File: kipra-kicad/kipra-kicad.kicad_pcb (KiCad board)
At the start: 2 copper layers, 128.2 x 134.8 mm, 51 parts

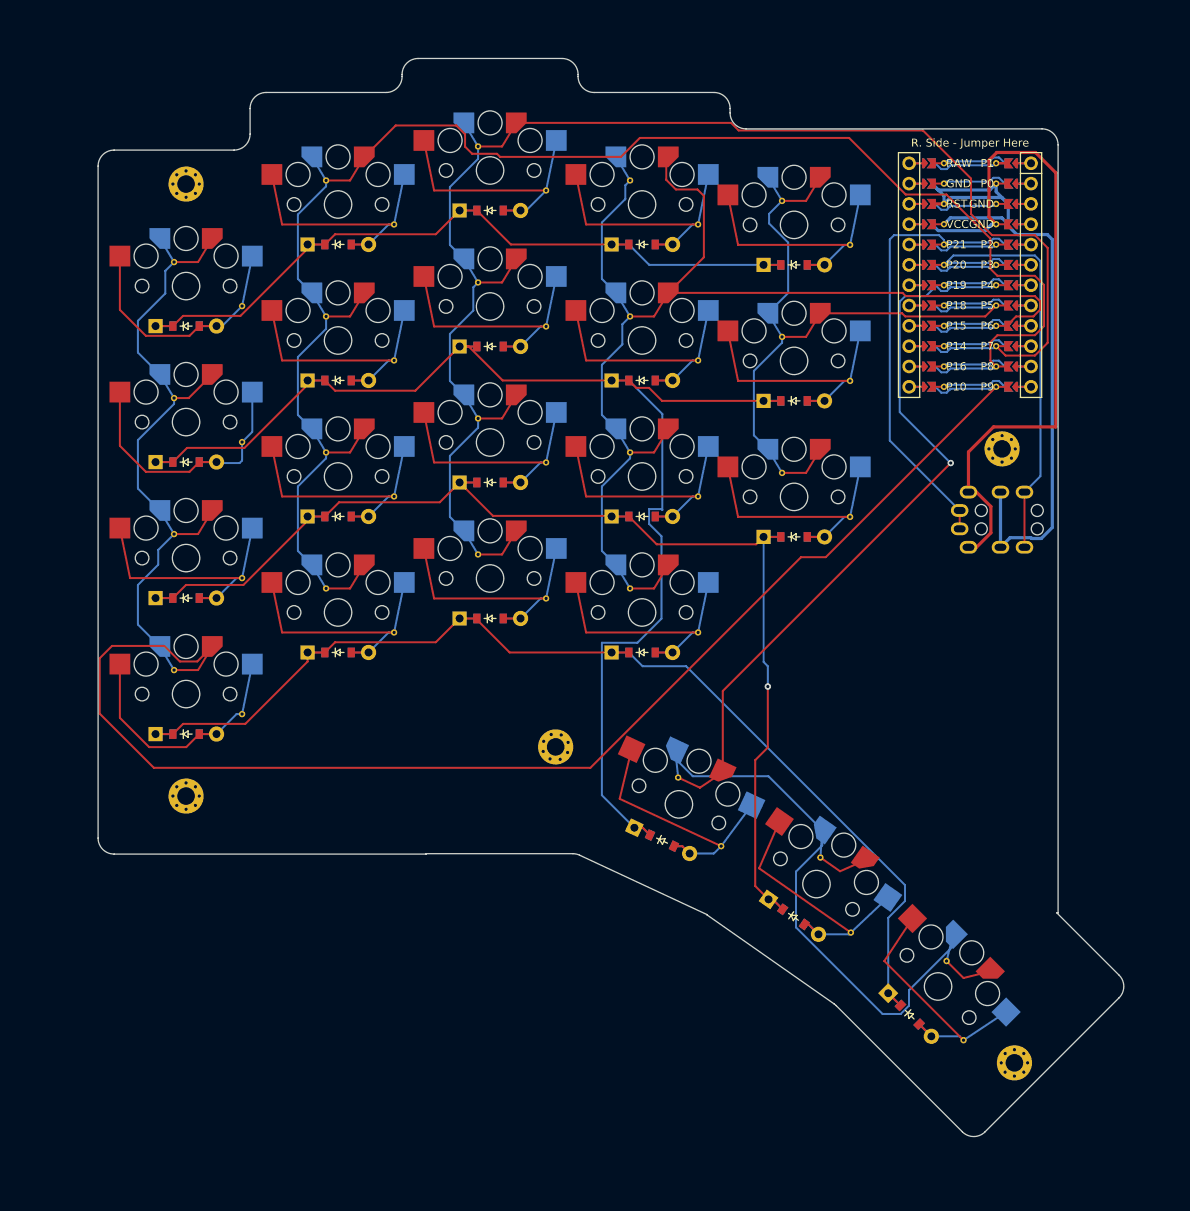
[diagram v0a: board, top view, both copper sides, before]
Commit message: DRC passes!
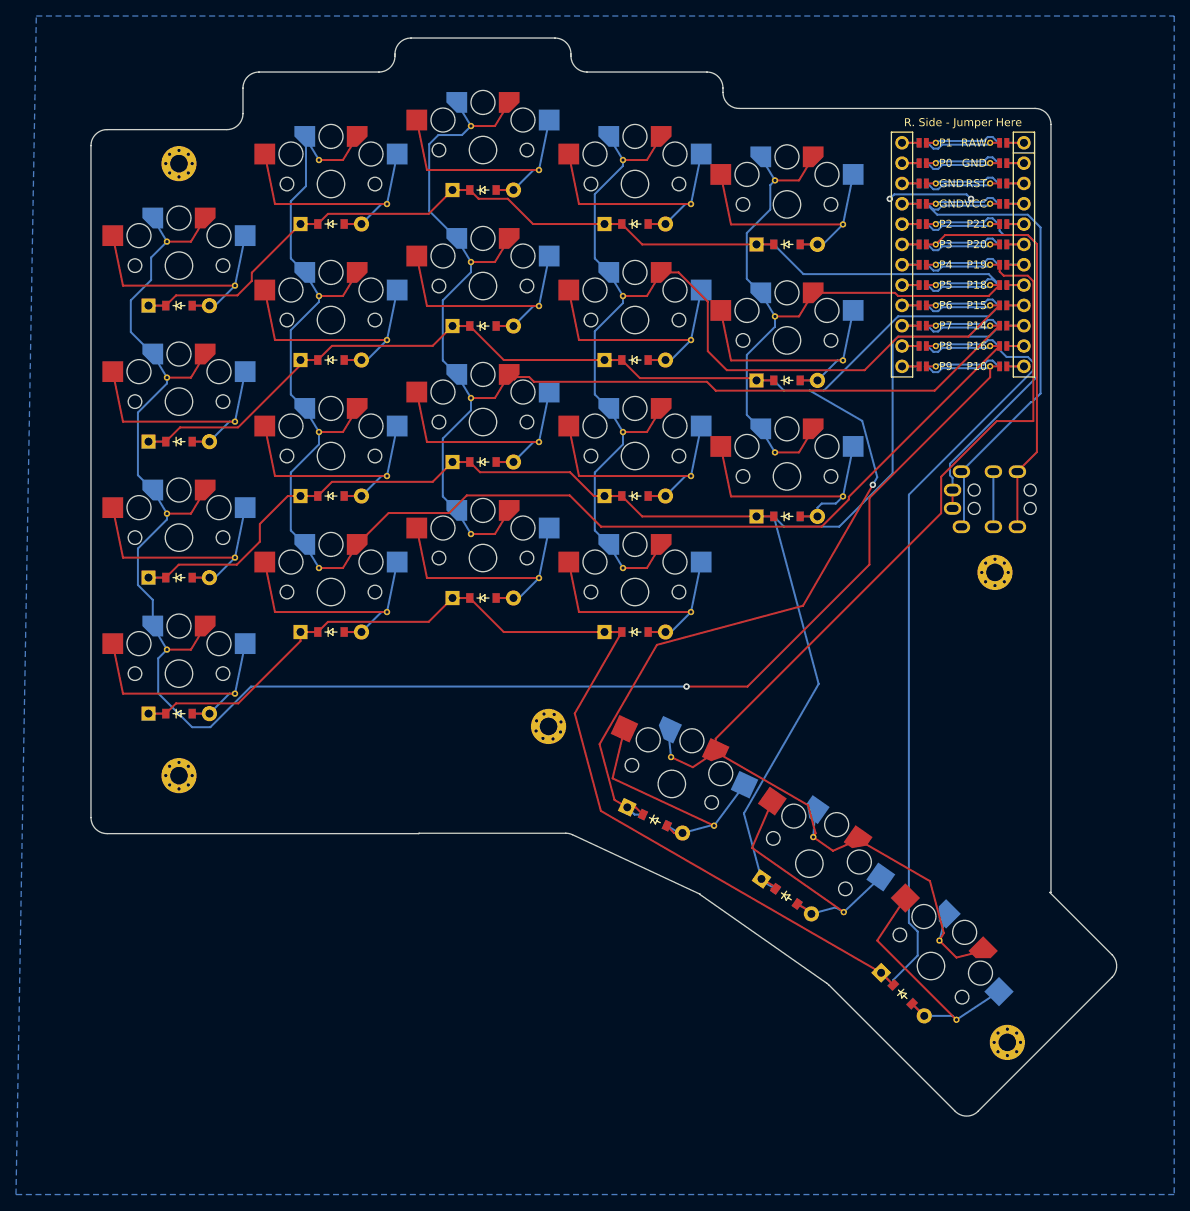
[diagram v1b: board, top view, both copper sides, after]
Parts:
- MCU1: footprint nice_nano -> ceoloide:nice_nano
- moved _3 15.5 mm to (201.1, 84.8)
- moved D16 2.71 mm to (156.1, 41.2)
- moved MCU1 2.71 mm to (197.1, 43.8)
- moved D11 2.71 mm to (137.1, 54.0)
- moved D15 2.71 mm to (156.1, 58.2)
- moved D2 2.71 mm to (99.1, 85.4)
- moved S17 2.71 mm to (175.1, 72.8)
- moved S6 2.71 mm to (118.1, 70.2)
- moved S3 2.71 mm to (99.1, 63.4)
- moved S4 2.71 mm to (99.1, 46.4)
- moved D7 2.71 mm to (118.1, 58.2)
- moved S16 2.71 mm to (156.1, 36.2)
- moved _1 2.71 mm to (99.1, 110.2)
- moved S12 2.71 mm to (137.1, 32.0)
- moved _2 2.71 mm to (99.1, 33.7)
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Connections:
- MCU1 pad 13: MCU1_13 -> MCU1_12
- MCU1 pad 14: MCU1_14 -> MCU1_11
- MCU1 pad 15: MCU1_15 -> MCU1_10
- MCU1 pad 16: MCU1_16 -> MCU1_9
- MCU1 pad 17: MCU1_17 -> MCU1_8
- MCU1 pad 18: MCU1_18 -> MCU1_7
- MCU1 pad 19: MCU1_19 -> MCU1_6
- MCU1 pad 20: MCU1_20 -> MCU1_5
- MCU1 pad 21: MCU1_21 -> MCU1_4
- MCU1 pad 22: MCU1_22 -> MCU1_3
- MCU1 pad 23: MCU1_23 -> MCU1_2
- MCU1 pad 24: MCU1_24 -> MCU1_1
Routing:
- net P8: track 151.7 -> 246.3 mm
- net GND: track 96.4 -> 46.4 mm, vias 0 -> 2
- net P7: track 162.6 -> 211.3 mm, vias 1 -> 0
- net P6: track 183.6 -> 221.6 mm, vias 0 -> 1
- net P5: track 108.2 -> 138.3 mm
- net P19: track 185.2 -> 158.5 mm, vias 1 -> 0
- net P14: track 193.4 -> 166.8 mm
- net P10: track 258.3 -> 234.9 mm, vias 0 -> 1
- net VCC: track 87.8 -> 67.0 mm
- net P16: track 214.4 -> 194.2 mm
- net P15: track 167.4 -> 152.2 mm
- net P2: track 57.8 -> 53.5 mm
- net RAW: track 11.7 -> 9.63 mm
- net pinky_one: track 33.8 -> 35.3 mm
- net pinky_four: track 34.2 -> 35.3 mm
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- added copper zone on B.Cu, net GND
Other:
- outline, holes or cut-outs redrawn
